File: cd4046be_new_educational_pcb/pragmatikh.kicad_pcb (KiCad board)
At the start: 2 copper layers, 44.5 x 32 mm, 10 parts, among them IC1 CD4046BE, J1 Conn_01x02_Socket, J2 Conn_01x08_Socket, J3 Conn_01x08_Socket, J4 Conn_01x02_Socket, J5 Conn_01x02_Socket, J6 Conn_01x02_Socket, J7 Conn_01x02_Socket, J8 Conn_01x02_Socket, J9 Conn_01x02_Socket

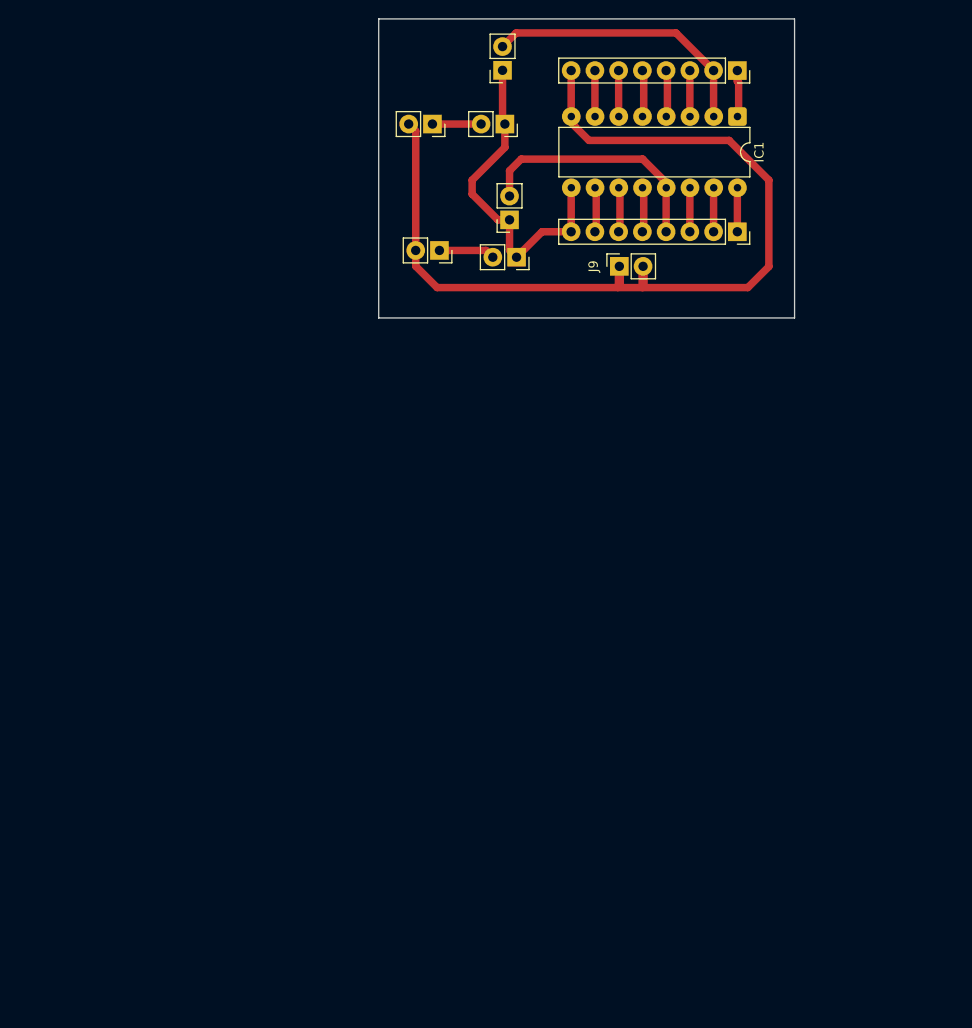
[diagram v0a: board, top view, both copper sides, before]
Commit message: l
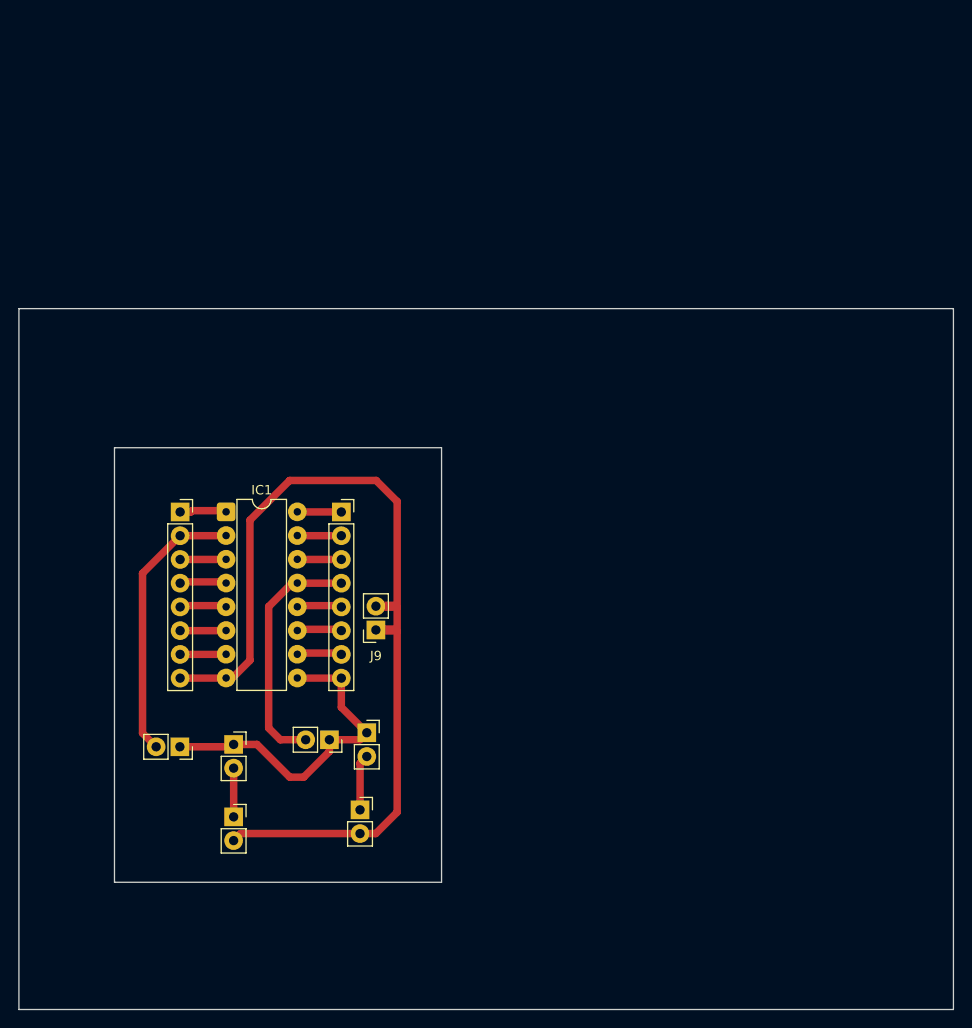
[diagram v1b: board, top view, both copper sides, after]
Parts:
- moved J1 80.2 mm to (112.2, 119.4), turned to -90 degrees
- moved J5 77.1 mm to (118.0, 126.9), turned to 0 degrees
- moved J2 76.1 mm to (112.2, 94.3), turned to 0 degrees
- moved J4 72.5 mm to (118.0, 119.1), turned to 0 degrees
- moved IC1 69.2 mm to (117.2, 94.2), turned to 0 degrees
- moved J7 60.5 mm to (131.5, 126.1), turned to 0 degrees
- moved J6 58.9 mm to (128.2, 118.6), turned to -90 degrees
- moved J8 53.3 mm to (132.2, 117.9), turned to 0 degrees
- moved J3 51.9 mm to (129.5, 94.3), turned to 0 degrees
- moved J9 46.8 mm to (133.2, 106.9), turned to 180 degrees
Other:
- board size 44.5 x 32 mm -> 100 x 75 mm
